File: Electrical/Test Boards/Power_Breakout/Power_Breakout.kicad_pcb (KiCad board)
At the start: 2 copper layers, 60.2 x 24 mm, 17 parts, among them P1 Header, Q1 FQP47P06, SW1 GF-123-0054, U1 LM2594

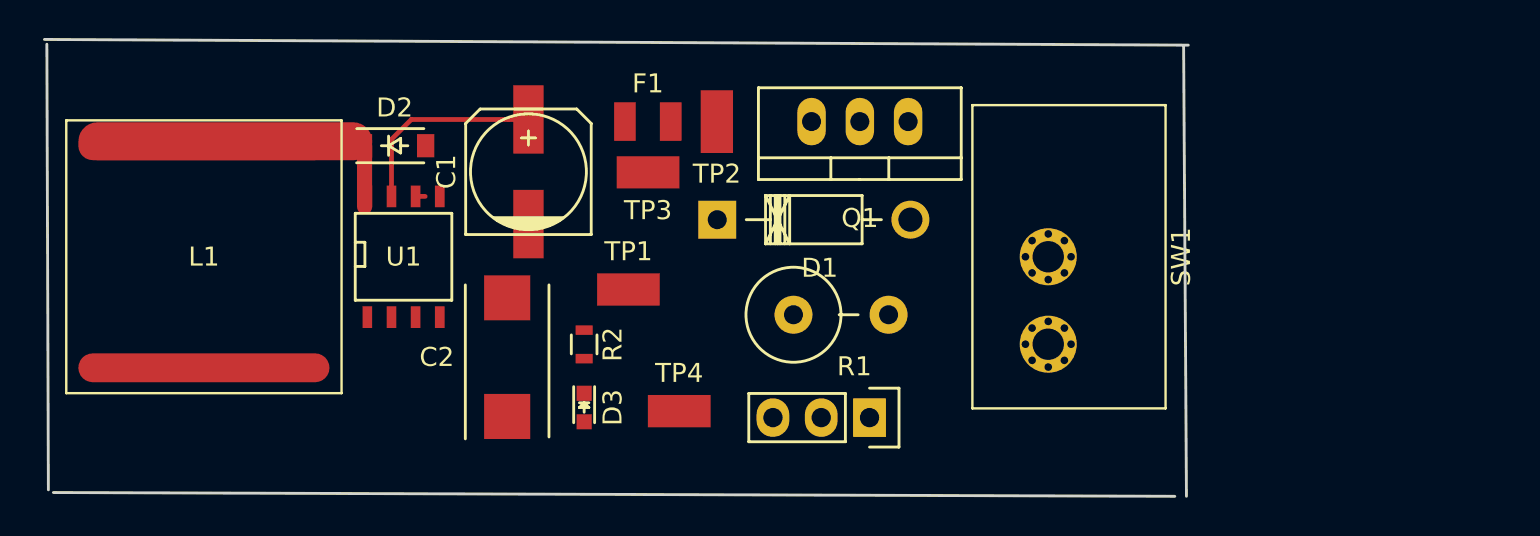
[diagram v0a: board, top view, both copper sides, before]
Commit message: Test board updates
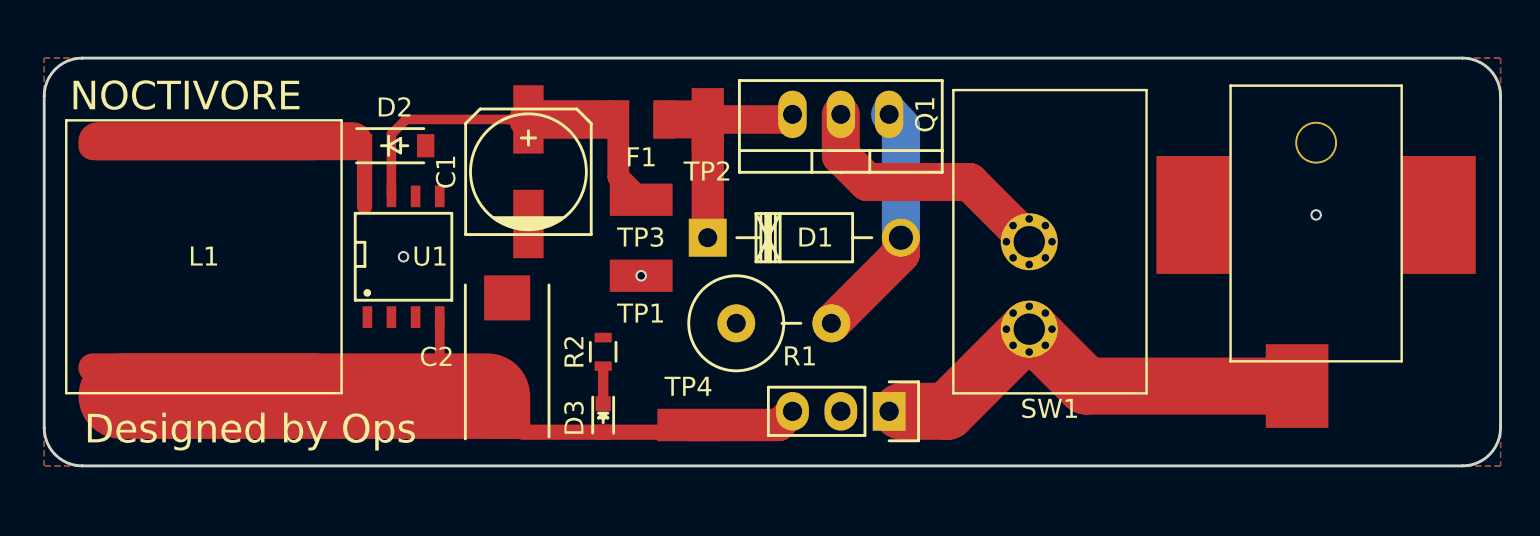
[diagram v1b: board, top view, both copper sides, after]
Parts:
- added CON1: BARREL_JACK, power_breakout:PJ-036AH-SMT-TR_Barrel_Jack, F.Cu at (178.0, 91.0)
- moved R1 3.04 mm to (150.0, 103.5)
- moved TP3 1.48 mm to (142.5, 97.0)
- moved SW1 1.28 mm to (164.0, 99.2)
- moved D3 1.14 mm to (140.5, 108.5)
- moved P1 1.08 mm to (155.5, 108.1)
- moved R2 1.07 mm to (140.5, 105.0)
- moved D1 1.07 mm to (146.0, 99.0)
- moved Q1 1.07 mm to (153.0, 92.5)
- moved TP1 0.98 mm to (142.5, 101.0)
- moved TP4 0.88 mm to (145.0, 108.8)
- moved TP2 0.49 mm to (146.0, 92.8)
- moved F1 0.37 mm to (142.5, 92.8)
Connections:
- U1 pad 1: (no net) -> GND
- U1 pad 2: (no net) -> GND
- U1 pad 3: (no net) -> GND
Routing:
- net +3V3: track 0.00 -> 37.5 mm
- net /VIN: track 0.00 -> 23.9 mm
- net Net-(Q1-Pad2): track 0.00 -> 14.0 mm
- net Net-(D1-Pad2): track 0.00 -> 12.7 mm
- net Net-(D1-Pad1): track 0.00 -> 12.3 mm
- net Net-(C1-Pad1): track 10.6 -> 19.8 mm
- net Net-(D3-Pad1): track 0.00 -> 1.93 mm
- net GND: track 0.50 -> 0.00 mm, vias 0 -> 3
- added copper zone on B.Cu, net GND
- added copper zone on F.Cu, net GND
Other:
- board size 60.2 x 24 mm -> 76.6 x 21.5 mm
- board text added: "Designed by Ops"
- board text added: "NOCTIVORE"
